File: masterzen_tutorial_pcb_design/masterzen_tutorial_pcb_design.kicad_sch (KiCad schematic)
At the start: 27 parts, among them SW85 SW_SPDT, U1 AMS1117, U3 PRTR5V0U2X, U4 STM32F303RETx, Y1 16MHz

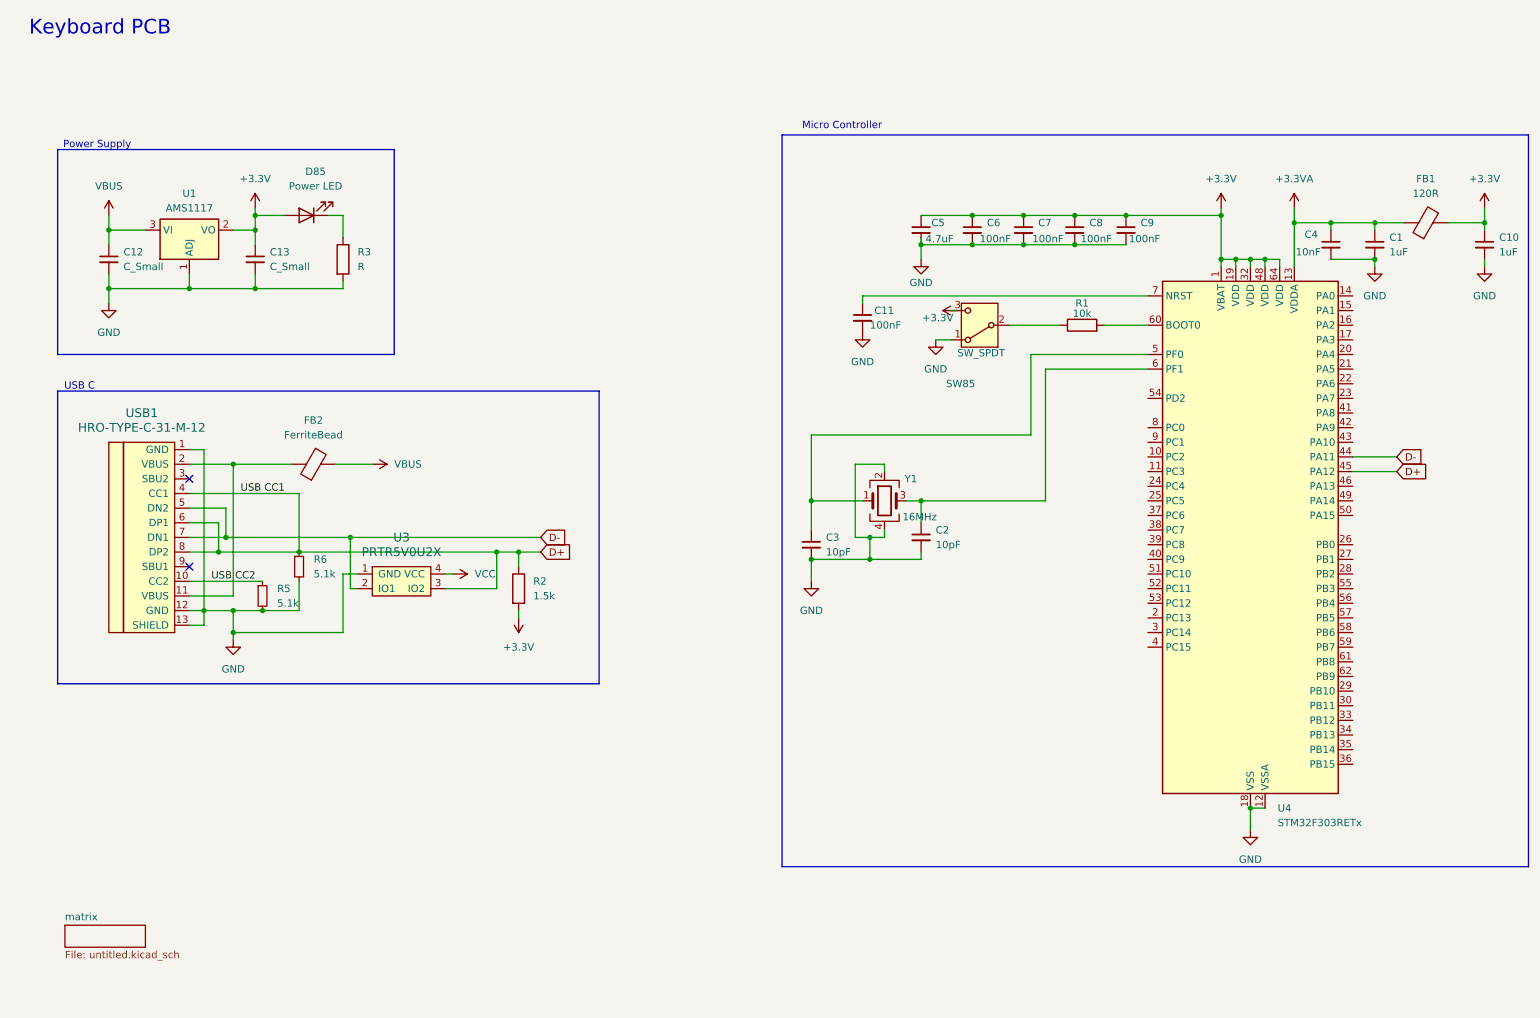
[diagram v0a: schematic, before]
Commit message: finished schematic
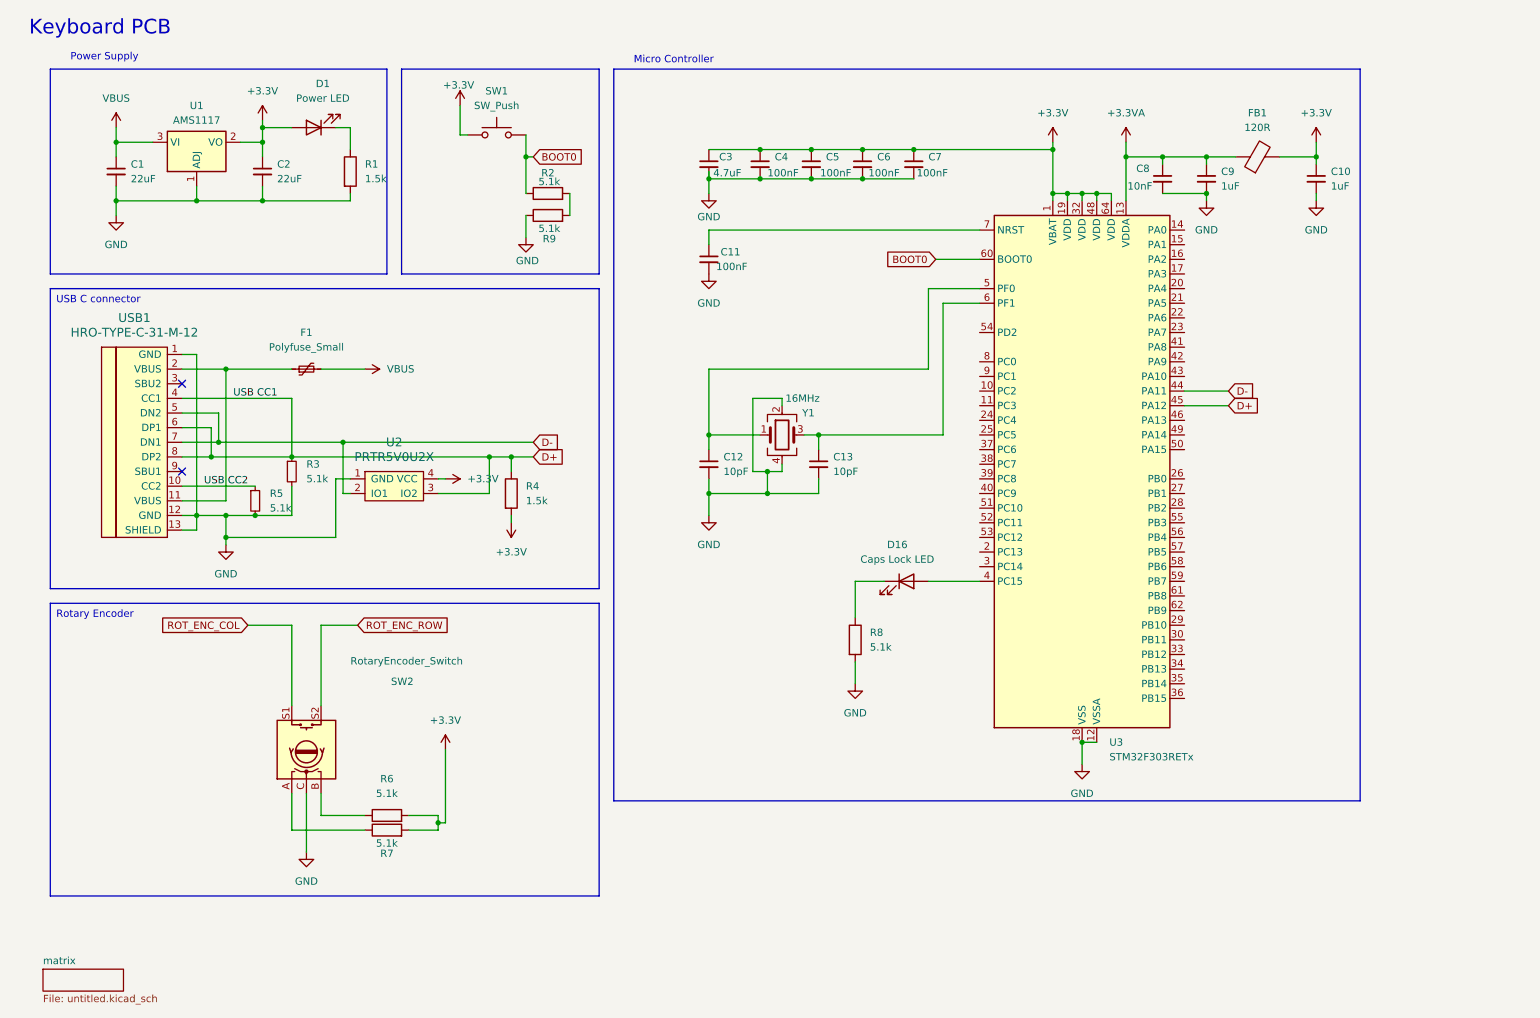
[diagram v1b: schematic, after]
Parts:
- removed FB2: FerriteBead, symbol Device:FerriteBead
- removed R1: 10k, symbol Device:R
- removed SW85: SW_SPDT, symbol Switch:SW_SPDT
- added D16: Caps Lock LED, symbol Device:LED
- added F1: Polyfuse_Small, Fuse:Fuse_0805_2012Metric_Pad1.15x1.40mm_HandSolder, symbol Device:Polyfuse_Small
- added R2, R8, R9: 5.1k, symbol Device:R
- added R6, R7: 5.1k, Resistor_SMD:R_0805_2012Metric_Pad1.20x1.40mm_HandSolder, symbol Device:R
- added SW1: SW_Push, Button_Switch_SMD:SW_SPST_SKQG_WithStem, symbol Switch:SW_Push
- added SW2: RotaryEncoder_Switch, Rotary_Encoder:RotaryEncoder_Alps_EC11E-Switch_Vertical_H20mm_CircularMountingHoles, symbol Device:RotaryEncoder_Switch
- C1: renamed from C12; value C_Small -> 22uF; footprint (none) -> Capacitor_SMD:C_0805_2012Metric_Pad1.18x1.45mm_HandSolder
- C10, C11: footprint (none) -> Capacitor_SMD:C_0805_2012Metric_Pad1.18x1.45mm_HandSolder
- C12: renamed from C3; footprint (none) -> Capacitor_SMD:C_0805_2012Metric_Pad1.18x1.45mm_HandSolder
- C13: renamed from C2; footprint (none) -> Capacitor_SMD:C_0805_2012Metric_Pad1.18x1.45mm_HandSolder
- C2: renamed from C13; value C_Small -> 22uF; footprint (none) -> Capacitor_SMD:C_0805_2012Metric_Pad1.18x1.45mm_HandSolder
- C3: renamed from C5; footprint (none) -> Capacitor_SMD:C_0805_2012Metric_Pad1.18x1.45mm_HandSolder
- C4: renamed from C6; footprint (none) -> Capacitor_SMD:C_0805_2012Metric_Pad1.18x1.45mm_HandSolder
- C5: renamed from C7; footprint (none) -> Capacitor_SMD:C_0805_2012Metric_Pad1.18x1.45mm_HandSolder
- C6: renamed from C8; footprint (none) -> Capacitor_SMD:C_0805_2012Metric_Pad1.18x1.45mm_HandSolder
- C7: renamed from C9; footprint (none) -> Capacitor_SMD:C_0805_2012Metric_Pad1.18x1.45mm_HandSolder
- C8: renamed from C4; footprint (none) -> Capacitor_SMD:C_0805_2012Metric_Pad1.18x1.45mm_HandSolder
- C9: renamed from C1; footprint (none) -> Capacitor_SMD:C_0805_2012Metric_Pad1.18x1.45mm_HandSolder
- D1: renamed from D85; footprint (none) -> LED_SMD:LED_0201_0603Metric_Pad0.64x0.40mm_HandSolder
- FB1: footprint (none) -> Ferrite_THT:LairdTech_28C0236-0JW-10
- R1: renamed from R3; value R -> 1.5k; footprint (none) -> Resistor_SMD:R_0805_2012Metric_Pad1.20x1.40mm_HandSolder
- R3: renamed from R6; footprint (none) -> Resistor_SMD:R_0805_2012Metric_Pad1.20x1.40mm_HandSolder
- R4: renamed from R2; footprint (none) -> Resistor_SMD:R_0805_2012Metric_Pad1.20x1.40mm_HandSolder
- R5: footprint (none) -> Resistor_SMD:R_0805_2012Metric_Pad1.20x1.40mm_HandSolder
- U2: renamed from U3; footprint (none) -> random-keyboard-parts:SOT143B
- USB1: footprint (none) -> Type-C:HRO-TYPE-C-31-M-12-HandSoldering
- Y1: footprint (none) -> Crystal:Crystal_SMD_3225-4Pin_3.2x2.5mm
- renumbered U4 to U3
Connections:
- net VCC is gone; now on net +3.3V: U2.4 (VCC)
- net +3.3V: now also R6.2, R7.2, SW1.1
- net GND: now also R8.2, R9.1, SW2.C
- net VBUS: now also F1.2
- net at U3.4 (PC15): now also D16.2 (A)
- net BOOT0: now reaches U3.60 (BOOT0)
- net BOOT0: now also R2.1, SW1.2
- net at USB1.11 (VBUS), USB1.2 (VBUS): now also F1.1
- new net: R6.1, SW2.B
- new net: D16.1 (K), R8.1
- new net: R2.2, R9.2
- new net: R7.1, SW2.A
- new net ROT_ENC_COL: SW2.S1
- new net ROT_ENC_ROW: SW2.S2
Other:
- note removed: "USB C"
- moved on the sheet: C1, C10, C11, C12, C13, C2, C3, C4, C5, C6, C7, C8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
